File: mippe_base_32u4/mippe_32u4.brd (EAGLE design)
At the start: 160 x 100 mm, 32 parts, among them J1 i2c, J2 USB, J3 spi, J4 i2c, J5 BURNIN, SW1 BTN-PTS810, U1 ATMEGA32U4-XUMU, Y1 16MHz

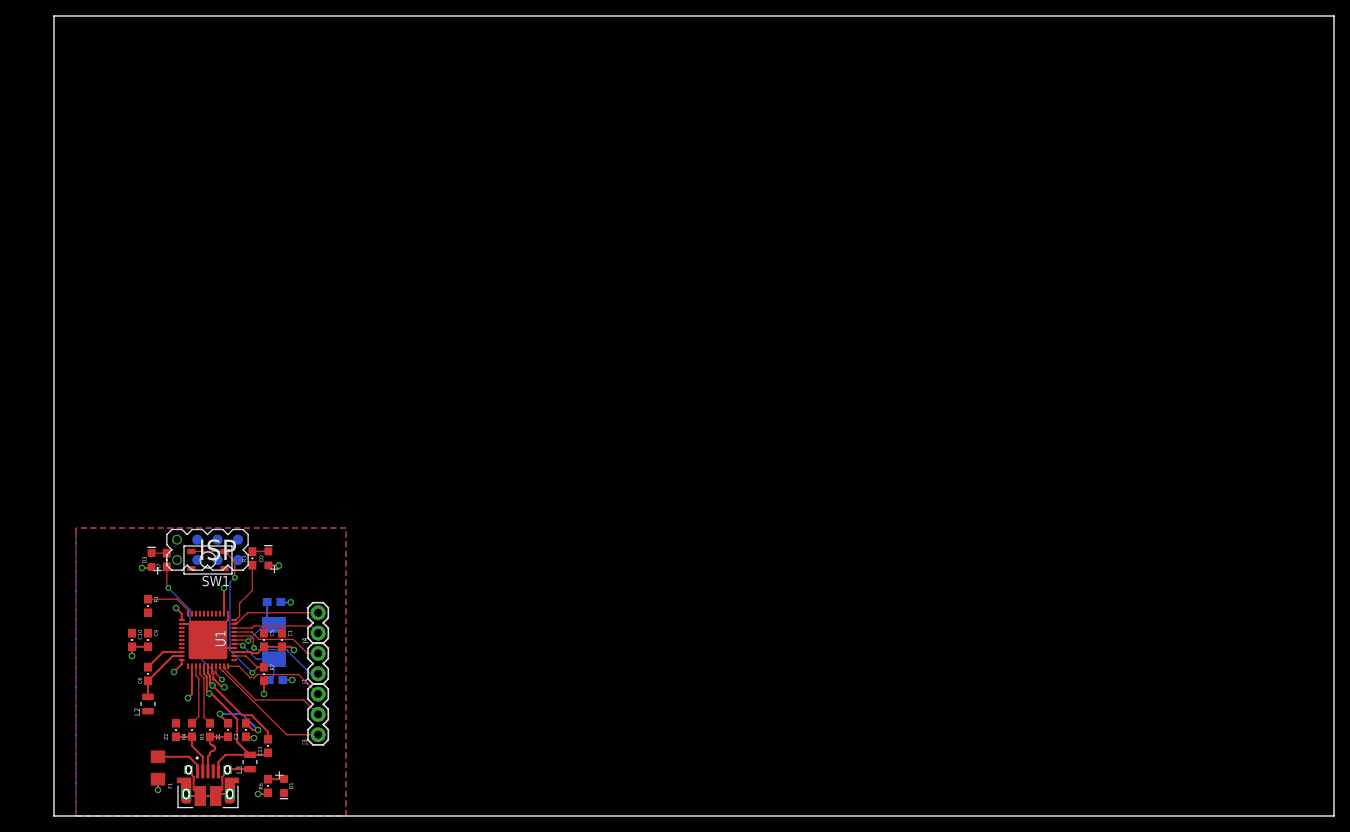
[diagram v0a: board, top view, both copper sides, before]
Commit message: finish 32u4 and rev c burnin
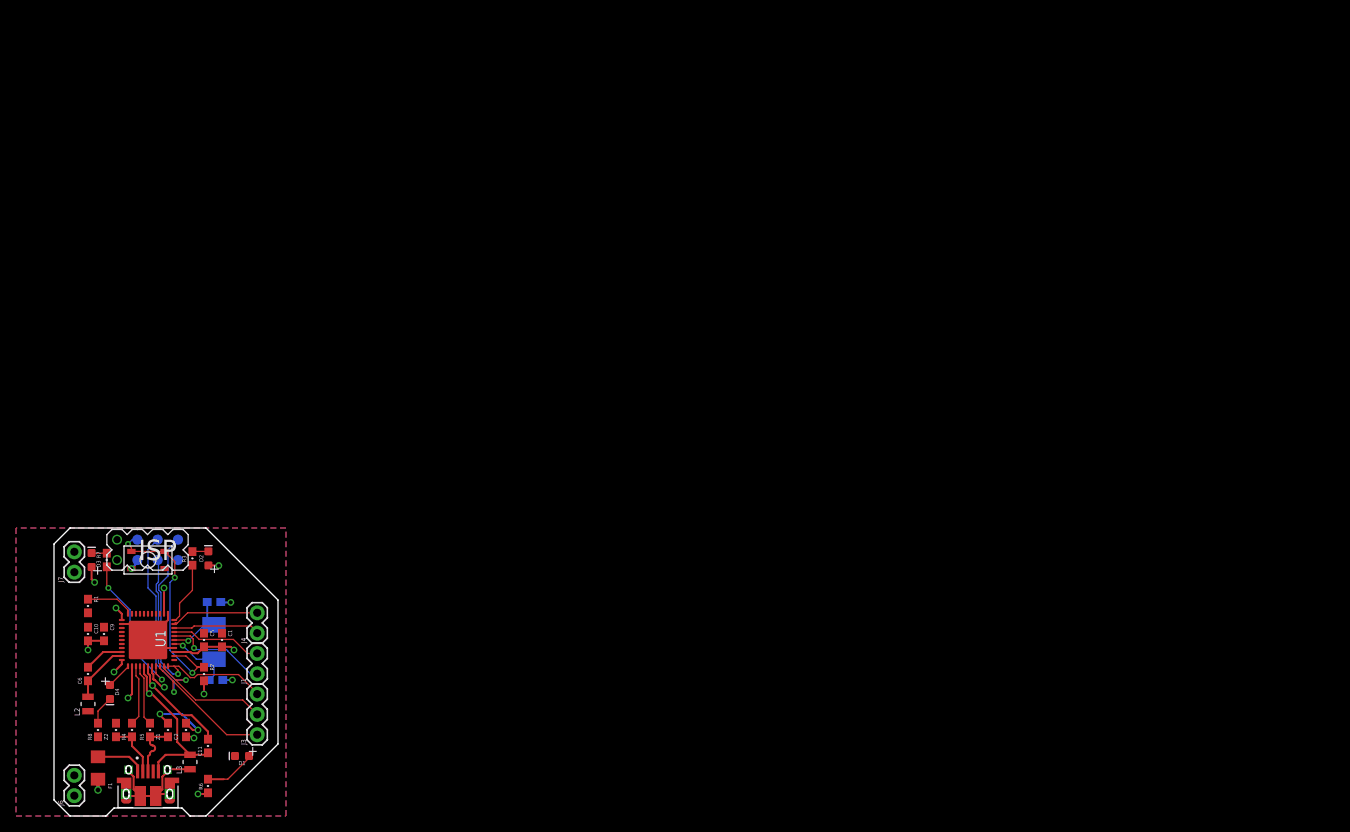
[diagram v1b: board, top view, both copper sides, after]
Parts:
- added D4: (no value), scono:LED-0603
- added J6: GND, scono:1X02
- added J7: VCC, scono:1X02
- added R8: 330R, scono:0603-RES
- J4: value i2c -> UART
- moved J1 7.62 mm to (25.4, 17.8)
- moved J3 7.62 mm to (25.4, 10.2)
- moved J4 7.62 mm to (25.4, 22.9)
- moved C1 7.50 mm to (21.0, 22.0)
- moved C11 7.50 mm to (19.2, 8.75)
- moved C2 7.50 mm to (16.5, 10.8)
- moved C3 7.50 mm to (20.0, 26.8)
- moved C4 7.50 mm to (20.2, 17.0)
- moved C5 7.50 mm to (18.8, 22.0)
- moved C6 7.50 mm to (4.25, 17.8)
- moved D2 7.50 mm to (19.3, 32.2)
- moved F1 7.50 mm to (5.50, 6.00)
- moved J2 7.50 mm to (11.8, 2.75)
- moved J5 7.50 mm to (15.5, 32.0)
- moved L2 7.50 mm to (4.25, 14.0)
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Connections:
- new net N$4: D4.C, R8.2
- net 5V: now also J5.3.3V, J7.1, J7.2
- net D7: now also D4.A
- net GND: now also J5.GND, J6.1, J6.2, R8.1
- net MISO: now also J5.MISO
- net MOSI: now also J5.MOSI
- net RESET: now also J5.RST
- net SCK: now also J5.SCK
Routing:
- net SCK: track 16.0 -> 38.2 mm, vias 0 -> 1
- net MISO: track 13.0 -> 33.5 mm, vias 0 -> 1
- net MOSI: track 14.4 -> 33.0 mm, vias 0 -> 1
- net N$3: track 2.01 -> 6.47 mm
- net N$4: track 0.00 -> 3.64 mm
- net D7: track 0.00 -> 3.28 mm
- net RESET: track 27.3 -> 29.8 mm, vias 2 -> 3
- net GND: track 23.6 -> 25.0 mm, vias 4 -> 5
- net 5V: track 33.7 -> 34.5 mm
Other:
- board size 160 x 100 mm -> 28 x 36 mm
- board text added: "Arias Research Group"
- board text added: "Design by Seiya Fa'19"
